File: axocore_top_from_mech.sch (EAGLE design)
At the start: 25 parts, among them X1 X1, X3 M02PTH, X4 M02PTH

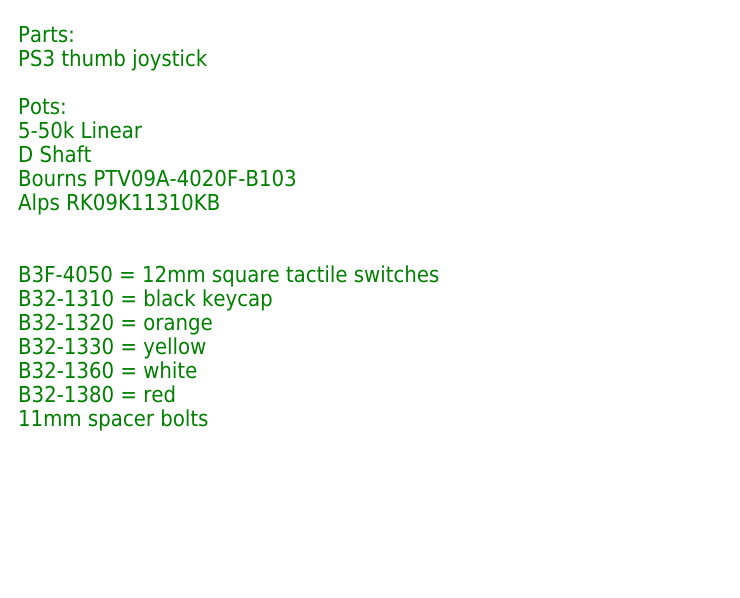
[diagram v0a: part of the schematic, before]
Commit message: Rev 1 Complete and sent to OSHPark
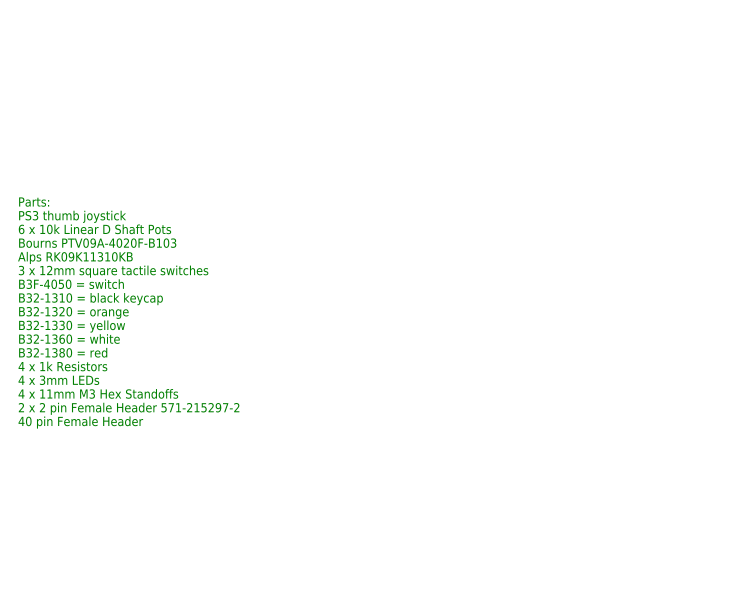
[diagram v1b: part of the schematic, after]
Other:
- note added: "Parts: PS3 thumb joystick 6 x 10k Linear D Shaft Pots Bourns PTV09A-4020F-B103 Alps RK09K11310KB 3 x 12mm square tactile switches B3F-4050 = switch B32-1310 = black keycap B32-1320 = orange B32-1330 = yellow B32-1360 = white B32-1380 = red 4 x 1k Resistors 4 x 3mm LEDs 4 x 11mm M3 Hex Standoffs 2 x 2 pin Female Header 571-215297-2 40 pin Female Header"
- note removed: "Parts: PS3 thumb joystick Pots: 5-50k Linear D Shaft Bourns PTV09A-4020F-B103 Alps RK09K11310KB B3F-4050 = 12mm square tactile switches B32-1310 = black keycap B32-1320 = orange B32-1330 = yellow B32-1360 = white B32-1380 = red 11mm spacer bolts"
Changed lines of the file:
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@@
 <sheet>
 <plain>
-<text x="-35.56" y="96.52" size="1.778" layer="91">Parts:
+<text x="-35.56" y="96.52" size="1.016" layer="91">Parts:
 PS3 thumb joystick
-Pots:
-5-50k Linear
-D Shaft
+6 x 10k Linear D Shaft Pots
 Bourns PTV09A-4020F-B103
 Alps RK09K11310KB
-B3F-4050 = 12mm square tactile switches
+3 x 12mm square tactile switches
+B3F-4050 = switch
 B32-1310 = black keycap
 B32-1320 = orange
@@
 B32-1360 = white
 B32-1380 = red
-11mm spacer bolts </text>
+4 x 1k Resistors
+4 x 3mm LEDs
+4 x 11mm M3 Hex Standoffs
+2 x 2 pin Female Header 571-215297-2
+40 pin Female Header</text>
 </plain>
 <instances>
